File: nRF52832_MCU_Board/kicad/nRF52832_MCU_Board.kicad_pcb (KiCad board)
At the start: 2 copper layers, 65 x 40 mm, 60 parts, among them J1 CONN_01X03, J2 CONN_01X16, J3 CONN_01X08, J4 CONN_01X03, J5 MICROUSB, J6 CONN_02X05, J7 CONN_01X05, J8 MM8130-2600, J9 CONN_01X08, SW1 SW_SPST, SW2 SW_SPST, U2 TLV1117, X1 32MHz, X2 32.768kHz

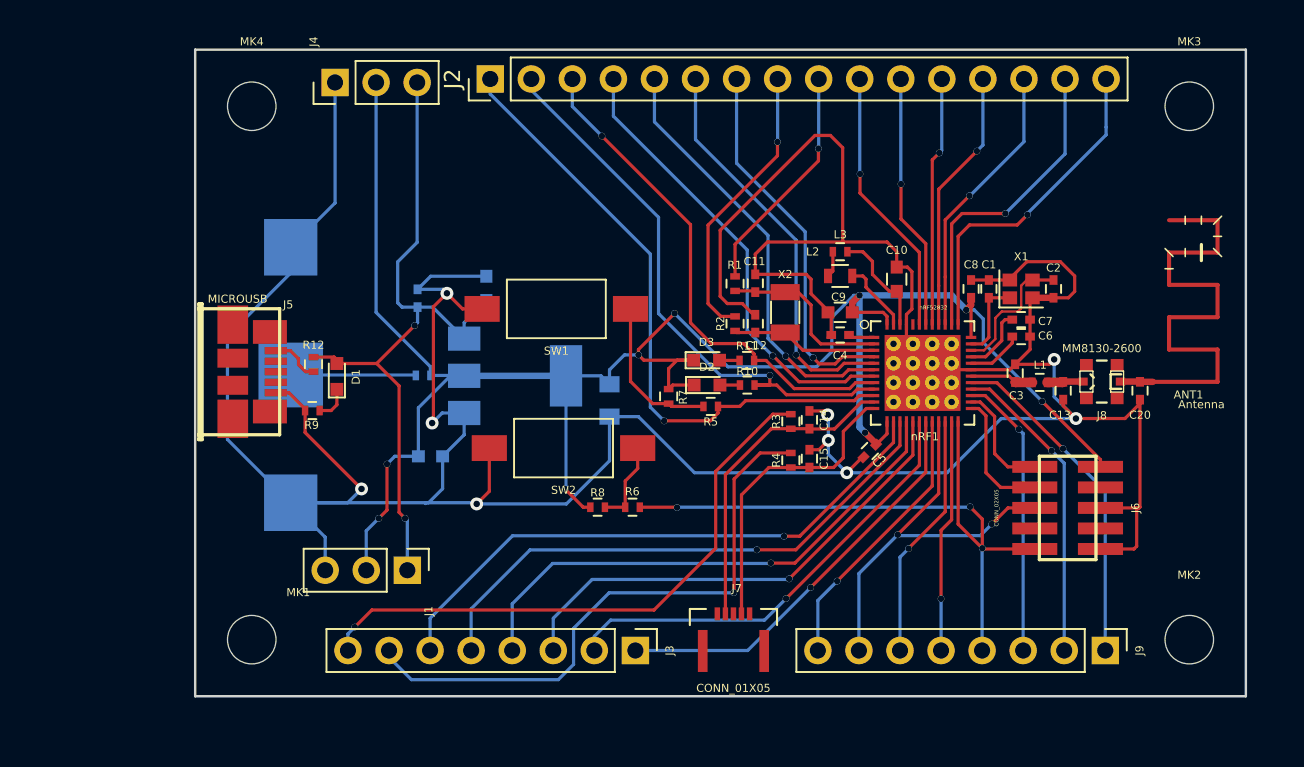
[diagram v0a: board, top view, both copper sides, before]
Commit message: Update KiCAD Project nRF52832_MCU_Board
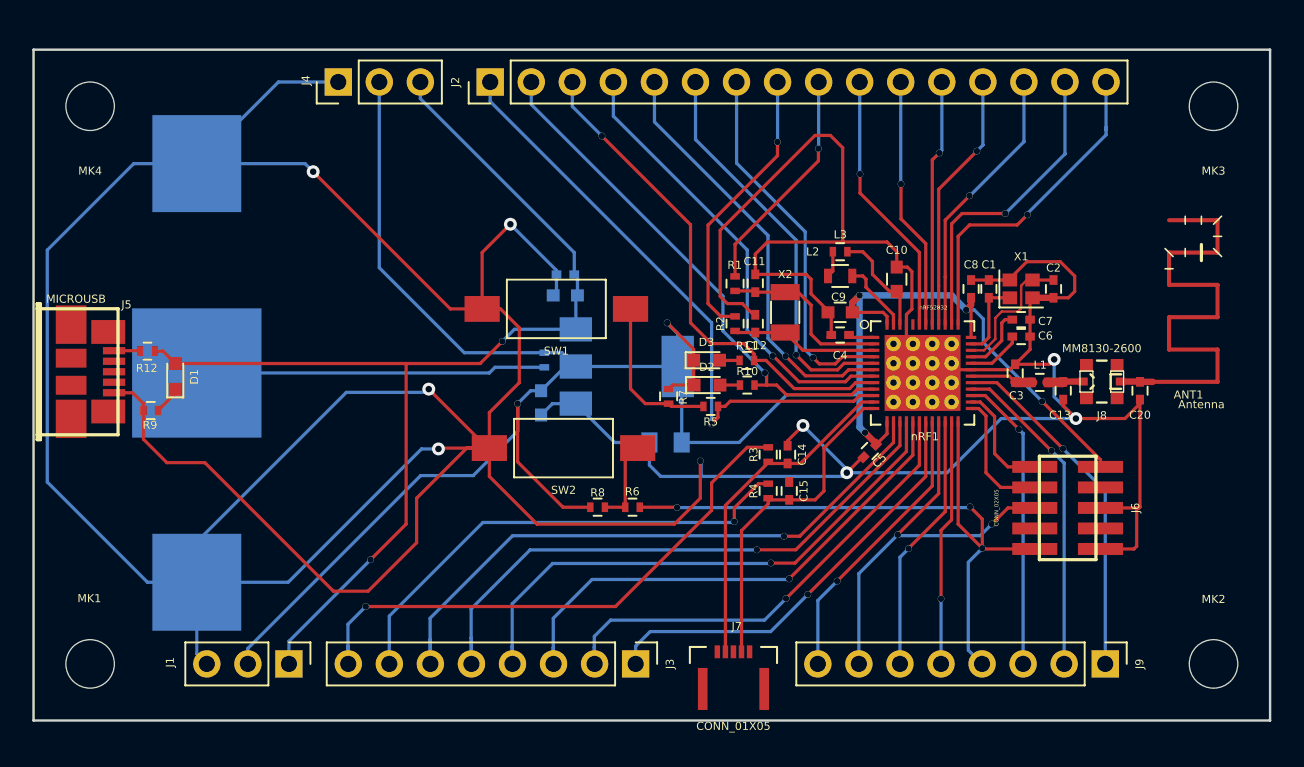
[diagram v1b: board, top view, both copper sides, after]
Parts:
- BATT1: value CR1632 -> CR2032; footprint w_battery_holders:keystone_3000 -> Nordic_misc:keystone_3003
- moved R12 10.3 mm to (52.0, 98.7), turned to 180 degrees
- moved MK1 10.1 mm to (48.5, 118.0)
- moved D1 10.0 mm to (53.8, 100.2)
- moved J5 10.0 mm to (47.3, 99.9)
- moved MK4 10.0 mm to (48.5, 83.5), turned to 180 degrees
- moved R9 10.0 mm to (52.2, 102.3)
- moved J1 9.34 mm to (60.8, 118.0)
- moved C16 9.26 mm to (77.9, 93.9), turned to 180 degrees
- moved C18 7.60 mm to (76.4, 101.8), turned to 270 degrees
- moved R13 7.56 mm to (76.6, 99.2), turned to 270 degrees
- moved U2 6.93 mm to (81.7, 99.6)
- moved BATT1 5.81 mm to (55.1, 100.0)
- moved C17 4.91 mm to (77.9, 95.2), turned to 180 degrees
- moved C19 4.33 mm to (84.1, 104.3), turned to 180 degrees
- moved C14 2.54 mm to (91.7, 105.0)
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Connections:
- J5 pad 2: (no net) -> Net-(J5-Pad2)
- J5 pad 3: (no net) -> Net-(J5-Pad3)
- J5 pad 4: (no net) -> Net-(J5-Pad4)
- J6 pad 4: (no net) -> Net-(J6-Pad4)
- J6 pad 7: (no net) -> Net-(J6-Pad7)
- J6 pad 8: (no net) -> Net-(J6-Pad8)
- J7 pad 1: (no net) -> Net-(J7-Pad1)
- J7 pad 3: (no net) -> Net-(J7-Pad3)
- J7 pad 5: (no net) -> Net-(J7-Pad5)
- nRF1 pad 44: (no net) -> Net-(nRF1-Pad44)
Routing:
- net GND: track 276.5 -> 378.4 mm
- net +5V: track 44.4 -> 68.2 mm
- net +3.3VP: track 7.75 -> 21.6 mm
- net +3V3: track 125.6 -> 136.5 mm, vias 9 -> 6
- net /P0.10: track 37.1 -> 30.3 mm
- net /P0.09: track 36.8 -> 34.3 mm
- net /P0.07: track 35.6 -> 33.3 mm
- net /nRF528323_MCU/NFC2: track 18.7 -> 20.7 mm
- net /P0.12: track 34.8 -> 36.4 mm
- net /P0.21: track 41.4 -> 43.0 mm
- net /P0.11: track 36.5 -> 38.0 mm
- net /P0.08: track 39.5 -> 38.0 mm
- net +5VD: track 3.08 -> 1.63 mm
- net /P0.16: track 25.7 -> 26.8 mm
- net /P0.13: track 33.0 -> 34.1 mm
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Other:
- board size 65 x 40 mm -> 76.5 x 41.5 mm
